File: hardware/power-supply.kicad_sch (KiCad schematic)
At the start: 19 parts, among them Q3 AO3401A, U3 LM5164DDA, U4 TPS7A0533PDBZ

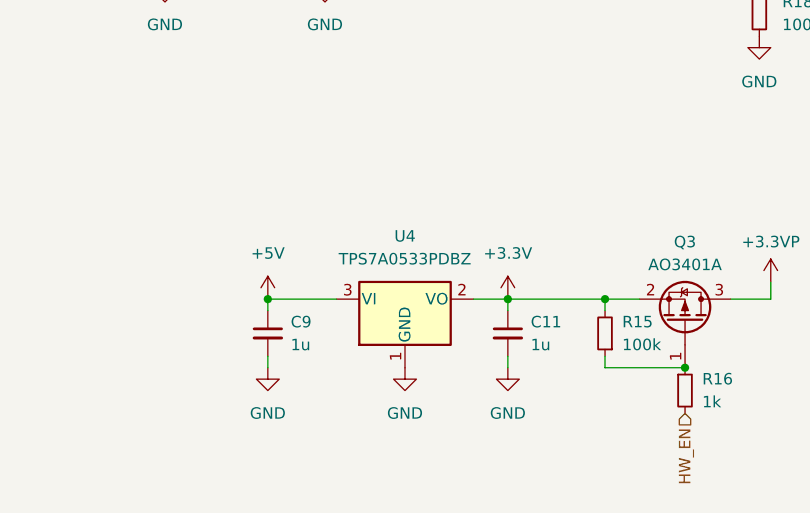
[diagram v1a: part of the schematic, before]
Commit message: ESP32 Decoupling
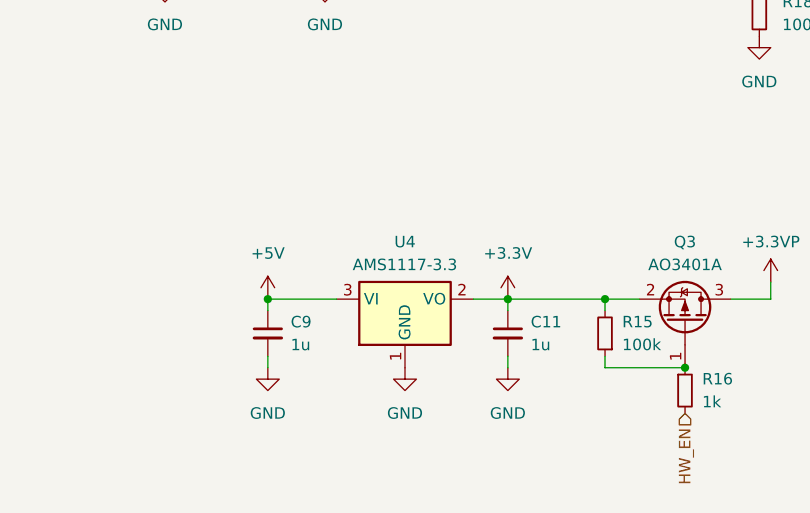
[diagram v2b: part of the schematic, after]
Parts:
- removed U4: TPS7A0533PDBZ, Package_TO_SOT_SMD:SOT-23, symbol Regulator_Linear:TPS7A0533PDBZ
- added U4: AMS1117-3.3, Package_TO_SOT_SMD:SOT-223-3_TabPin2, symbol Regulator_Linear:AMS1117-3.3
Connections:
- net +3.3V: now also U4.2 (VO)
- net +5V: now also U4.3 (VI)
- net GND: now also U4.1 (GND)
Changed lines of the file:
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@@
-	)
-	(symbol
-		(lib_id "Regulator_Linear:TPS7A0533PDBZ")
-		(at 130.81 110.49 0)
-		(unit 1)
-		(exclude_from_sim no)
-		(in_bom yes)
-		(on_board yes)
-		(dnp no)
-		(fields_autoplaced yes)
-		(property "Reference" "U4"
-			(at 130.81 103.505 0)
-			(effects
-				(font
-					(size 1.27 1.27)
-				)
-			)
-		)
-		(property "Value" "TPS7A0533PDBZ"
-			(at 130.81 106.045 0)
-			(effects
-				(font
-					(size 1.27 1.27)
-				)
-			)
-		)
-		(property "Footprint" "Package_TO_SOT_SMD:SOT-23"
-			(at 130.81 105.41 0)
-			(effects
-				(font
-					(size 1.27 1.27)
-				)
-				(hide yes)
-			)
-		)
-		(property "Datasheet" "https://www.ti.com/lit/ds/symlink/tps7a05.pdf"
-			(at 130.81 111.76 0)
-			(effects
-				(font
-					(size 1.27 1.27)
-				)
-				(hide yes)
-			)
-		)
-		(property "Description" ""
-			(at 130.81 110.49 0)
-			(effects
-				(font
-					(size 1.27 1.27)
-				)
-				(hide yes)
-			)
-		)
-		(pin "2"
-		)
-		(pin "1"
-		)
-		(pin "3"
-		)
-		(instances
-			(project "greenmobi-bms"
-				(path "/3e668e3e-3e16-4665-a807-4735962c41d3/600d3fd5-a2c8-411e-91ac-e4cbb4ace0f8"
-					(reference "U4")
-					(unit 1)
-				)
-			)
-		)
 	)
 	(symbol
@@
 					(unit 1)
 				)
+			)
+		)
+	)
+	(symbol
+		(lib_id "Regulator_Linear:AMS1117-3.3")
+		(at 130.81 110.49 0)
+		(unit 1)
+		(exclude_from_sim no)
+		(in_bom yes)
+		(on_board yes)
+		(dnp no)
+		(fields_autoplaced yes)
+		(property "Reference" "U4"
+			(at 130.81 104.14 0)
+			(effects
+				(font
+					(size 1.27 1.27)
+				)
+			)
+		)
+		(property "Value" "AMS1117-3.3"
+			(at 130.81 106.68 0)
+			(effects
+				(font
+					(size 1.27 1.27)
+				)
+			)
+		)
+		(property "Footprint" "Package_TO_SOT_SMD:SOT-223-3_TabPin2"
+			(at 130.81 105.41 0)
+			(effects
+				(font
+					(size 1.27 1.27)
+				)
+				(hide yes)
+			)
+		)
+		(property "Datasheet" "http://www.advanced-monolithic.com/pdf/ds1117.pdf"
+			(at 133.35 116.84 0)
+			(effects
+				(font
+					(size 1.27 1.27)
+				)
+				(hide yes)
+			)
+		)
+		(property "Description" "1A Low Dropout regulator, positive, 3.3V fixed output, SOT-223"
+			(at 130.81 110.49 0)
+			(effects
+				(font
+					(size 1.27 1.27)
+				)
+				(hide yes)
+			)
+		)
+		(pin "3"
+		)
+		(pin "2"
+		)
+		(pin "1"
+		)
+		(instances
+			(project ""
+				(path "/3e668e3e-3e16-4665-a807-4735962c41d3/600d3fd5-a2c8-411e-91ac-e4cbb4ace0f8"
+					(reference "U4")
+					(unit 1)
+				)
